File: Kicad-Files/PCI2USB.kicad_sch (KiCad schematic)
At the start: 1 part, among them J1 Bus_M.2_Socket_B

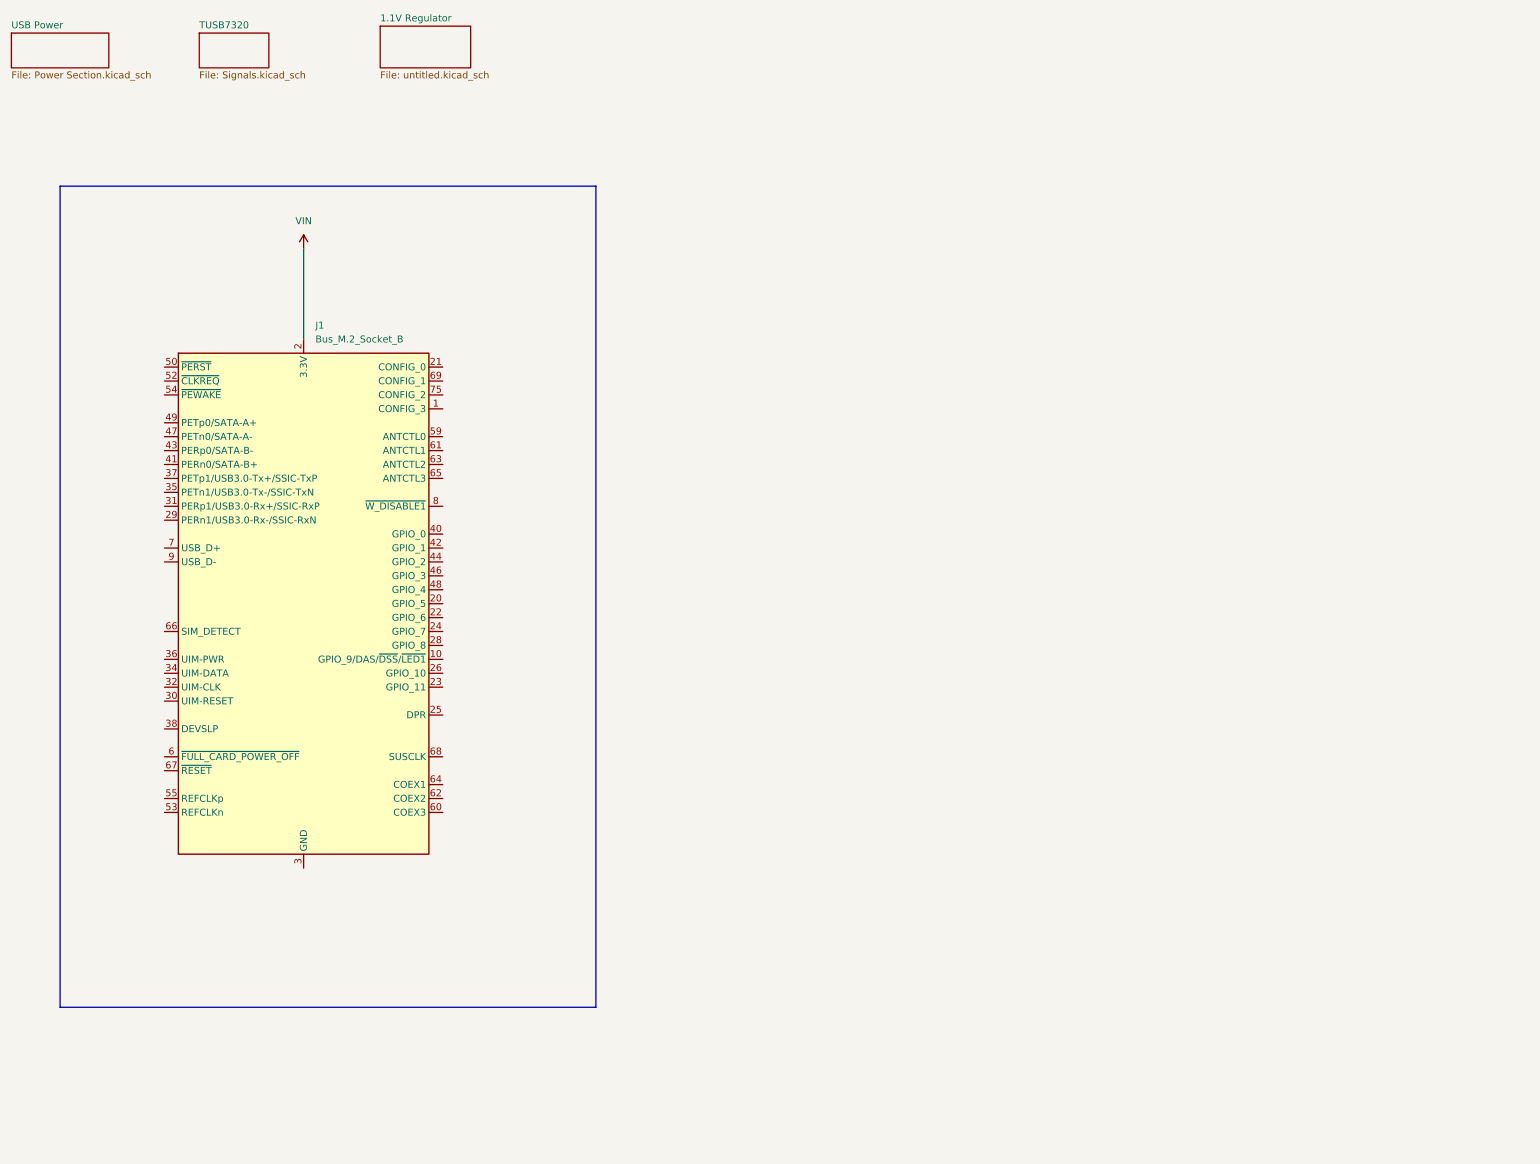
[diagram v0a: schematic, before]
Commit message: Created schematics for TUSB7320 USB Controller
Signed-off-by: Jakub Sobota <jakub.sobota@3mdeb.com>
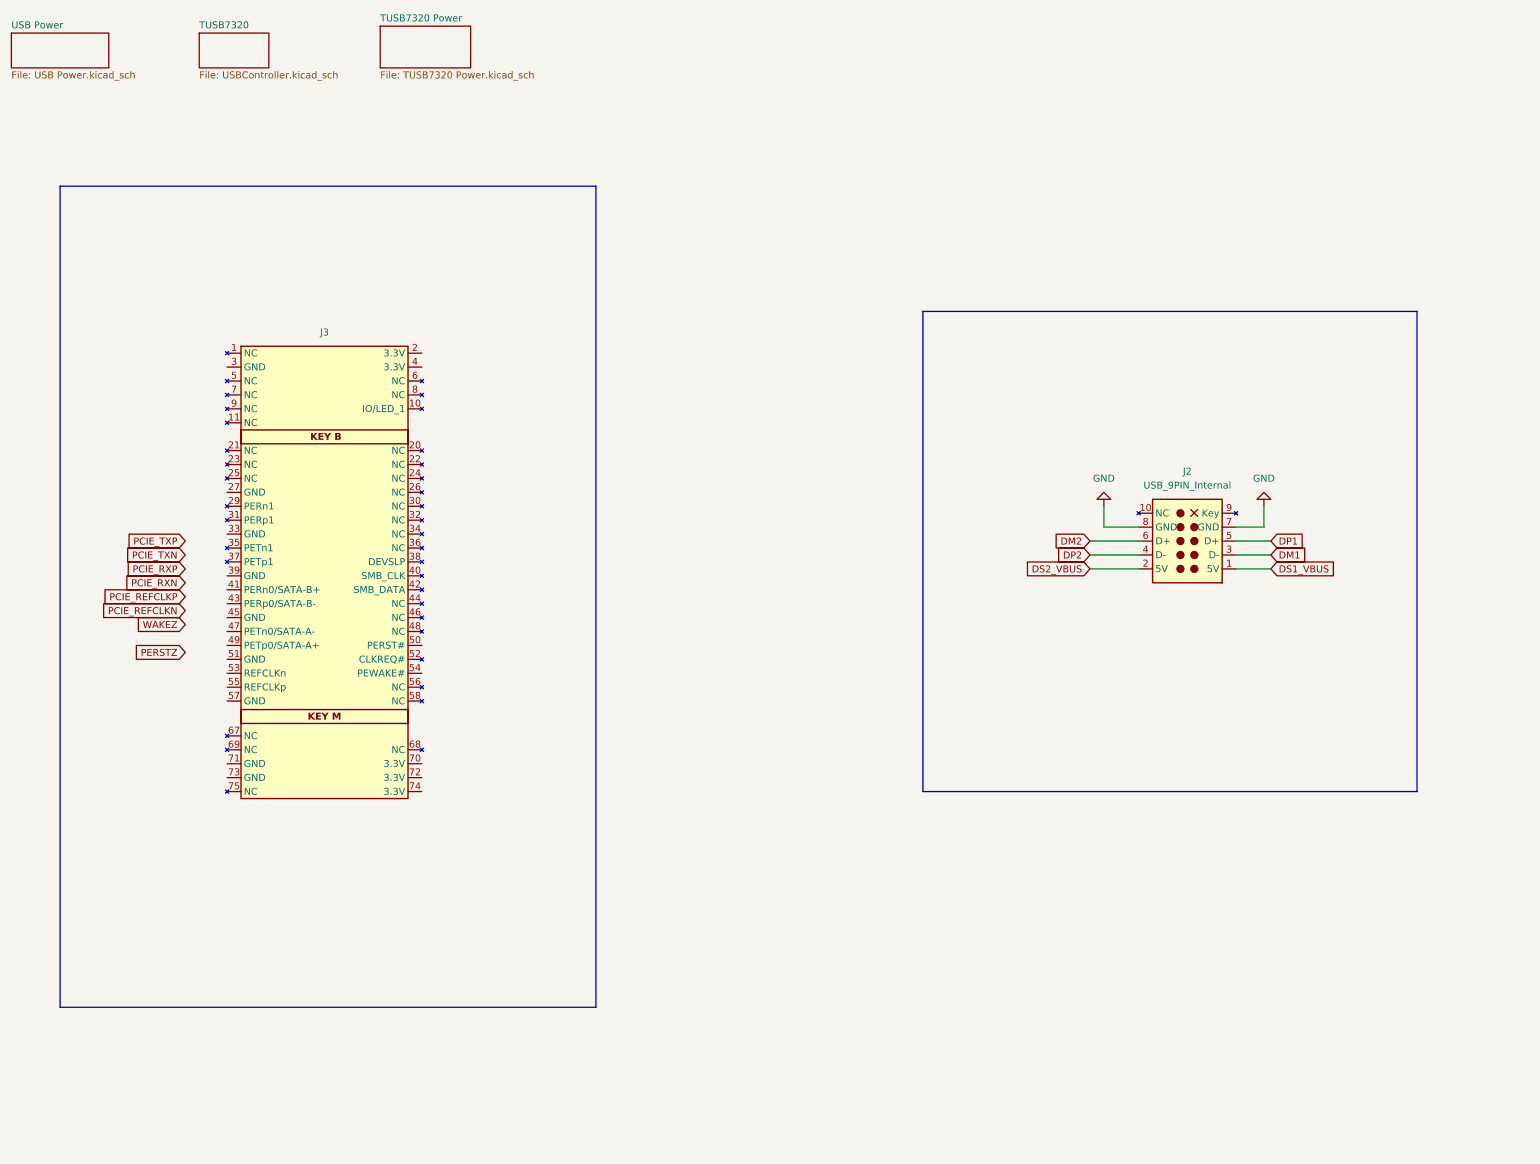
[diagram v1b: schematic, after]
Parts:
- removed J1: Bus_M.2_Socket_B, symbol Connector:Bus_M.2_Socket_B
- added J2: USB_9PIN_Internal, Connectors:USB 9 Pin internal header, symbol Connectors:USB_9PIN_Internal
- added J3: ~, M2_Edge_connector:M.2_KEY_M_B, symbol M2_Edge_connector:M.2_Key_M_B
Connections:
- new net DM1: J2.3 (D-)
- new net DM2: J2.6 (D+)
- new net DP1: J2.5 (D+)
- new net DP2: J2.4 (D-)
- new net DS1_VBUS: J2.1 (5V)
- new net DS2_VBUS: J2.2 (5V)
- new net GND: J2.7 (GND), J2.8 (GND)
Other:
- sheet 1.1V Regulator renamed TUSB7320 Power
- sheet TUSB7320: file Signals.kicad_sch -> USBController.kicad_sch
- sheet TUSB7320 Power: file untitled.kicad_sch -> TUSB7320 Power.kicad_sch
- sheet USB Power: file Power Section.kicad_sch -> USB Power.kicad_sch

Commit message: Complete Schematics and BOM
Signed-off-by: Jakub Sobota <jakub.sobota@3mdeb.com>
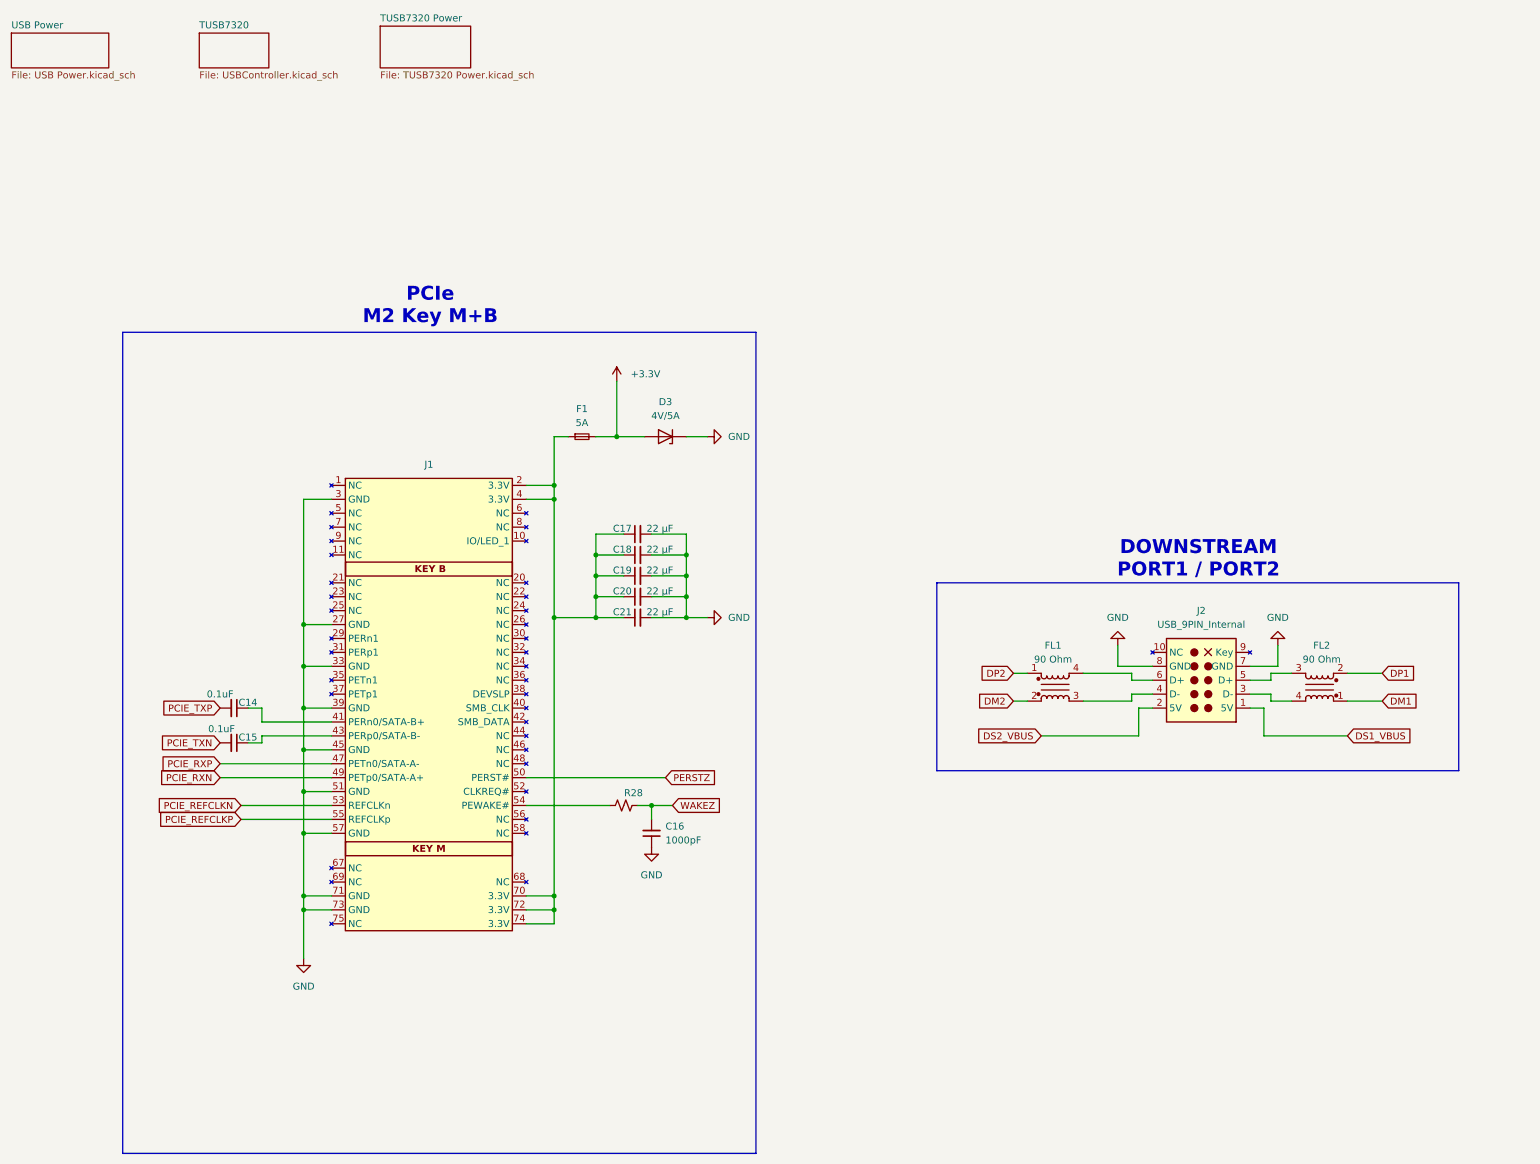
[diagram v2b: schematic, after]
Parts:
- added C14, C15: 0.1uF, Capacitor_SMD:C_0402_1005Metric_Pad0.74x0.62mm_HandSolder, symbol Device:C_Small
- added C16: 1000pF, Capacitor_SMD:C_0402_1005Metric_Pad0.74x0.62mm_HandSolder, symbol Device:C_Small
- added C17, C18, C19, C20, C21: 22 µF, Capacitor_SMD:C_0402_1005Metric_Pad0.74x0.62mm_HandSolder, symbol Device:C_Small
- added D3: 4V/5A, Diode_SMD:D_SOD-323_HandSoldering, symbol Diode:PTVS5V0Z1USK
- added F1: 5A, Fuse:Fuse_0603_1608Metric_Pad1.05x0.95mm_HandSolder, symbol Device:Fuse_Small
- added FL1, FL2: 90 Ohm, Filters:MCZ1210AH_CP, symbol Filter:Choke_CommonMode_PulseElectronics_PH9455x405NL
- added R28: 0 Ohm, Resistor_SMD:R_0402_1005Metric_Pad0.72x0.64mm_HandSolder, symbol Device:R_Small_US
- renumbered J3 to J1
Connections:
- net DM1: now also FL2.1; no longer J2.3 (D-)
- net DM2: now also FL1.2; no longer J2.6 (D+)
- net DP1: now also FL2.2; no longer J2.5 (D+)
- net DP2: now also FL1.1; no longer J2.4 (D-)
- net GND: now also J1.27 (GND), J1.3 (GND), J1.33 (GND), J1.39 (GND), J1.45 (GND), J1.51 (GND), J1.57 (GND), J1.71 (GND), J1.73 (GND), C16.1, C17.2, C18.2, C19.2, C20.2, C21.2, D3.1 (K)
- net PCIE_REFCLKN: now also J1.53 (REFCLKn)
- net PCIE_REFCLKP: now also J1.55 (REFCLKp)
- net PCIE_RXN: now also J1.49 (PETp0/SATA-A+)
- net PCIE_RXP: now also J1.47 (PETn0/SATA-A-)
- net PCIE_TXN: now also C15.2
- net PCIE_TXP: now also C14.2
- net PERSTZ: now also J1.50 (PERST#)
- net WAKEZ: now also C16.2, R28.1
- net at J1.2 (3.3V): now also J1.4 (3.3V), J1.70 (3.3V), J1.72 (3.3V), J1.74 (3.3V), C17.1, C18.1, C19.1, C20.1, C21.1, F1.1
- net at J1.41 (PERn0/SATA-B+): now also C14.1
- net at J1.43 (PERp0/SATA-B-): now also C15.1
- net at J1.54 (PEWAKE#): now also R28.2
- new net: FL2.3, J2.5 (D+)
- new net: FL2.4, J2.3 (D-)
- new net: FL1.3, J2.4 (D-)
- new net: FL1.4, J2.6 (D+)
- new net +3.3V: D3.2 (A), F1.2
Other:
- note added: "DOWNSTREAM PORT1 / PORT2"
- note added: "PCIe M2 Key M+B"
- company: 3mdeb Sp. z o.o -> 3mdeb Sp. z o.o    Jakub Sobota
- moved on the sheet: J1, J2

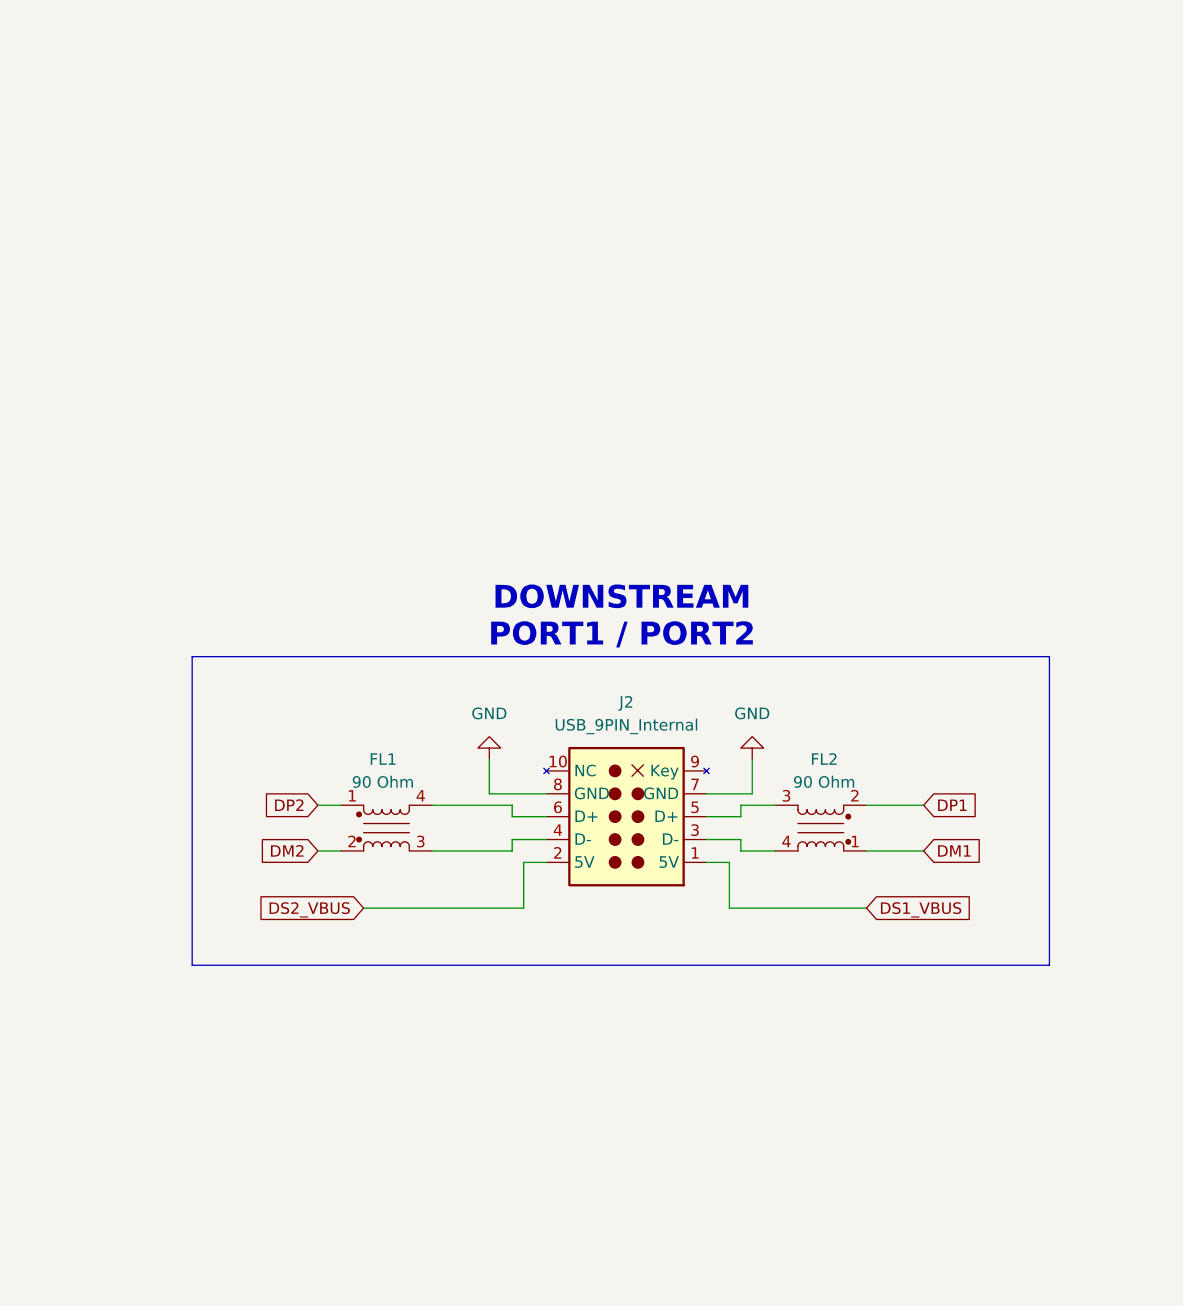
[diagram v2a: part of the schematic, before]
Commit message: Placed additional information to board schematics
Signed-off-by: Jakub Sobota <jakub.sobota@3mdeb.com>
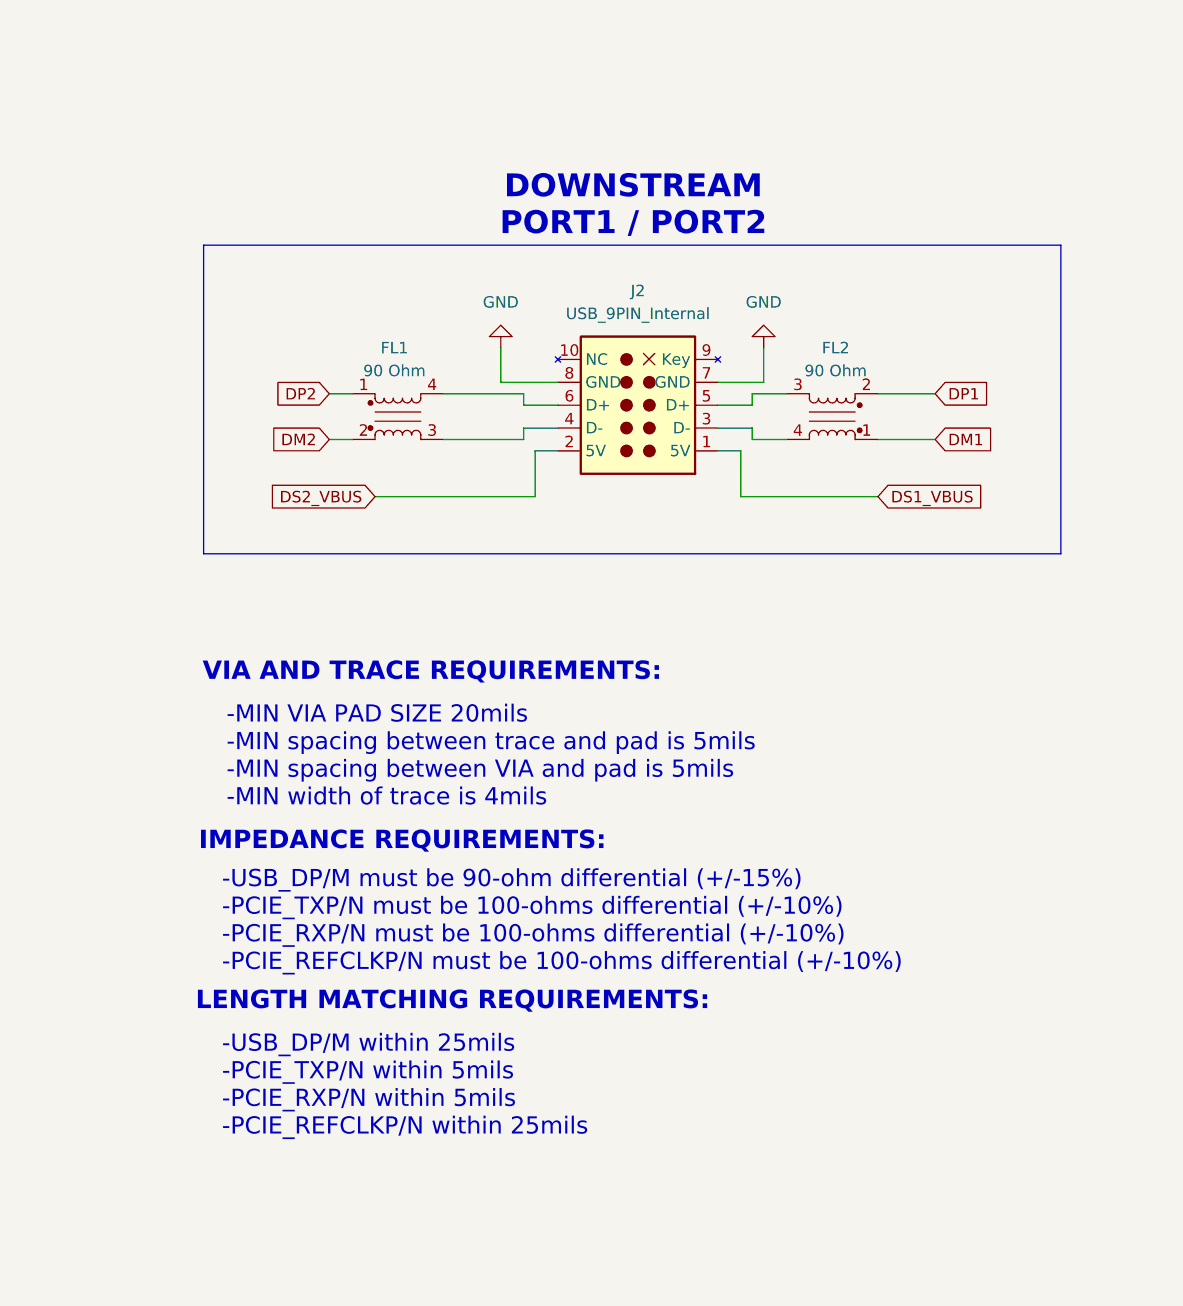
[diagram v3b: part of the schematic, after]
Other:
- note added: "-MIN VIA PAD SIZE 20mils -MIN spacing between trace and pad is 5mils -MIN spacing between VIA and pad is 5mils -MIN width of trace is 4mils"
- note added: "-USB_DP/M must be 90-ohm differential (+/-15%) -PCIE_TXP/N must be 100-ohms differential (+/-10%) -PCIE_RXP/N must be 100-ohms differential (+/-10%) -PCIE_REFCLKP/N must be 100-ohms differential (+/-10%)"
- note added: "-USB_DP/M within 25mils -PCIE_TXP/N within 5mils -PCIE_RXP/N within 5mils -PCIE_REFCLKP/N within 25mils"
- note added: "IMPEDANCE REQUIREMENTS:"
- note added: "LENGTH MATCHING REQUIREMENTS:"
- note added: "VIA AND TRACE REQUIREMENTS:"
- moved on the sheet: FL1, FL2, J2
